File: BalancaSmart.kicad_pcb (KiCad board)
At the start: 2 copper layers, 100 x 100 mm, 53 parts, among them J1 Load Cell, J2 Barrel_Jack, Q1 PMOS, Q2 NMOS, Q3 NMOS, Q4 S8050, SW1 SW_Push, U1 HX711-Mod, U2 ADS1115-module, U3 HX-2S-JH20, U4 XL4015

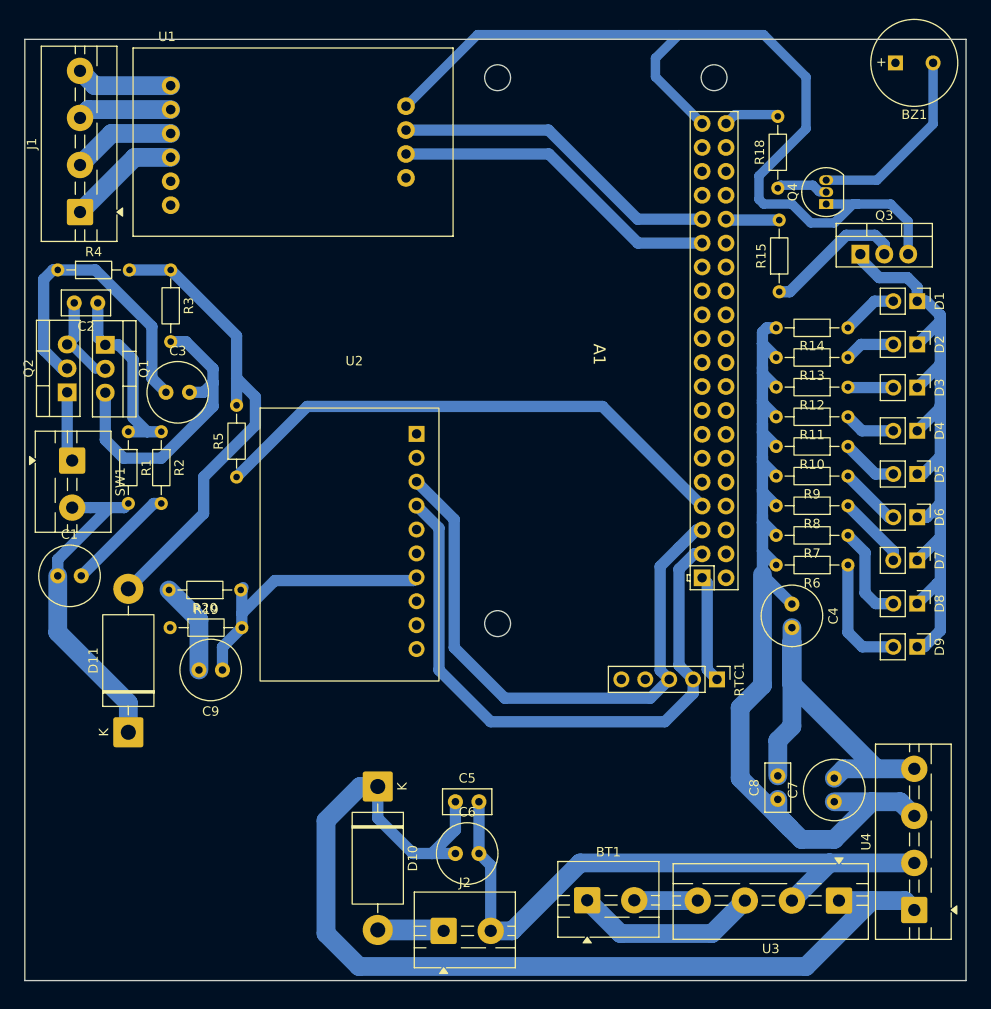
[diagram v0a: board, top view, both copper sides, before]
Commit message: layout PCB finalizado
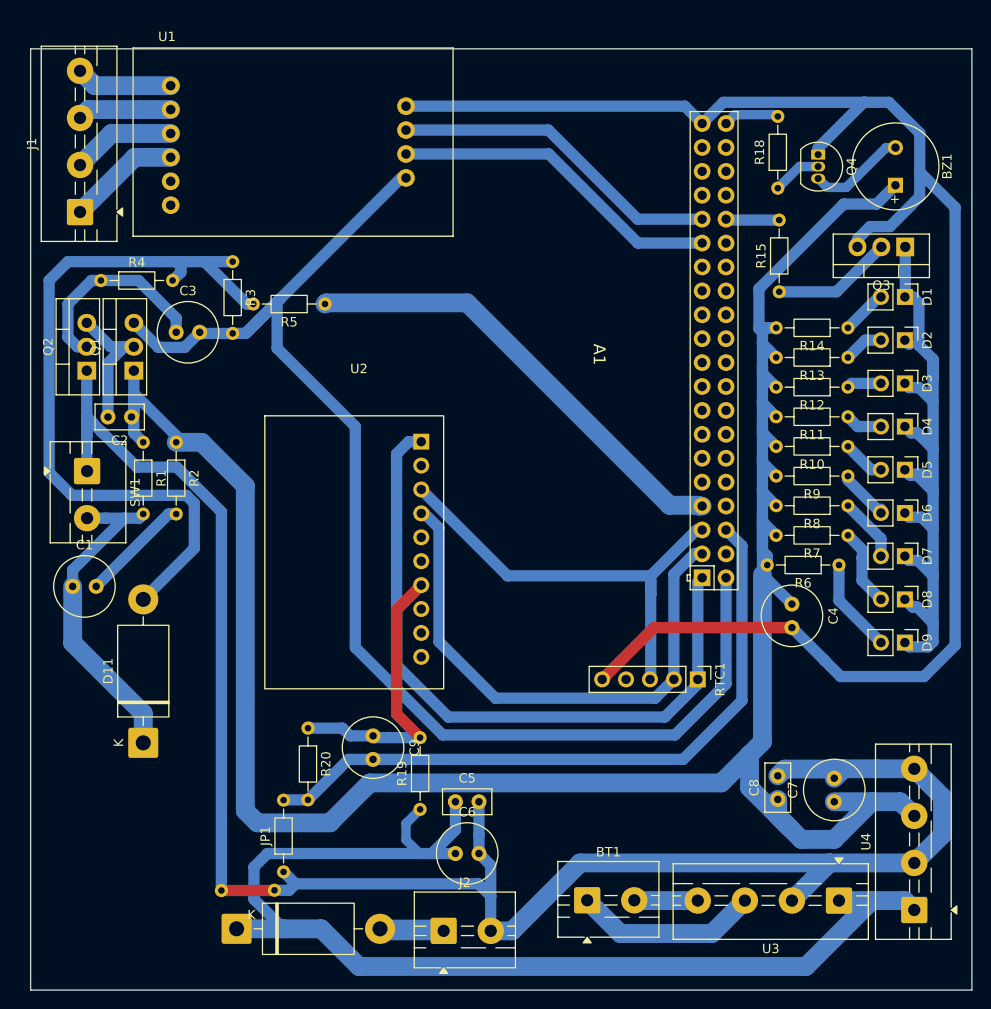
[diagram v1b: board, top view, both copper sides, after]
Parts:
- added ?: , , F.Cu at (83.4, 165.4)
- added ?: , , F.Cu at (89.0, 165.4)
- added JP1: Jumper_2_Bridged, Resistor_THT:R_Axial_DIN0204_L3.6mm_D1.6mm_P7.62mm_Horizontal, F.Cu at (90.0, 163.4)
- moved R19 32.8 mm to (104.5, 156.8), turned to 90 degrees
- moved D10 21.3 mm to (85.0, 169.5), turned to 0 degrees
- moved R5 20.6 mm to (94.4, 103.1), turned to 180 degrees
- moved C9 17.5 mm to (99.5, 149.0), turned to -90 degrees
- moved R20 16.3 mm to (92.6, 148.2), turned to -90 degrees
- moved BZ1 13.0 mm to (155.0, 90.5), turned to 90 degrees
- moved C2 12.6 mm to (73.8, 115.1)
- moved R3 6.64 mm to (84.6, 98.6)
- moved C3 6.47 mm to (78.6, 106.1)
- moved Q4 5.32 mm to (146.8, 87.2), turned to -90 degrees
- moved Q3 4.83 mm to (156.0, 97.0), turned to 180 degrees
- moved R4 4.72 mm to (70.6, 100.6)
- moved Q1 4.09 mm to (74.1, 110.2), turned to 90 degrees
- moved Q2 3.10 mm to (69.1, 110.2)
- moved RTC1 2.04 mm to (134.0, 143.0)
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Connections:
- A1 pad 6: unconnected-(A1-GND-Pad6) -> Earth
- C7 pad 2: Earth -> P-
- C8 pad 2: Earth -> P-
- Q2 pad 1: Earth -> P-
- SW1 pad 1: Earth -> P-
- U4 pad 4: Earth -> P-
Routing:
- net P-: track 67.9 -> 200.0 mm
- net +5V: track 128.9 -> 249.8 mm
- net pino 5v rasp: track 32.2 -> 140.1 mm
- net Earth: track 160.2 -> 248.5 mm
- net +3V3: track 11.4 -> 72.8 mm
- net Net-(D11-A): track 50.6 -> 79.6 mm
- net I2C SCL: track 63.6 -> 48.3 mm
- net P+: track 109.5 -> 122.8 mm
- net Net-(Q2-G): track 32.8 -> 21.6 mm
- net Net-(BZ1--): track 20.3 -> 10.4 mm
- net I2C SDA: track 65.9 -> 57.9 mm
- net Sinal de desligamento: track 57.0 -> 49.1 mm
- net Net-(Q1-G): track 9.85 -> 15.2 mm
- net Net-(D9-A): track 12.6 -> 10.1 mm
- net Net-(Q3-G): track 15.1 -> 12.8 mm
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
